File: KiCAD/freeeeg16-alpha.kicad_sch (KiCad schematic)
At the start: 27 parts, among them J1 Conn_02x03_Odd_Even, J2 Conn_01x03, J28 Conn_02x03_Odd_Even, J29 Conn_02x03_Odd_Even, J3 Conn_01x03, J30 Conn_02x03_Odd_Even, J31 Conn_02x03_Odd_Even, J32 Conn_02x03_Odd_Even, J33 Conn_02x03_Odd_Even, J5 Conn_01x08, J6 Conn_01x06, SW1 SW_Push, SW2 SW_Push, SW3 SW_Push, SW4 SW_Push

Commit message: Add files via upload
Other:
- moved on the sheet: C20, C39, C41, J1, J2, J3, J5, J6, R1, R10, R2, R4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

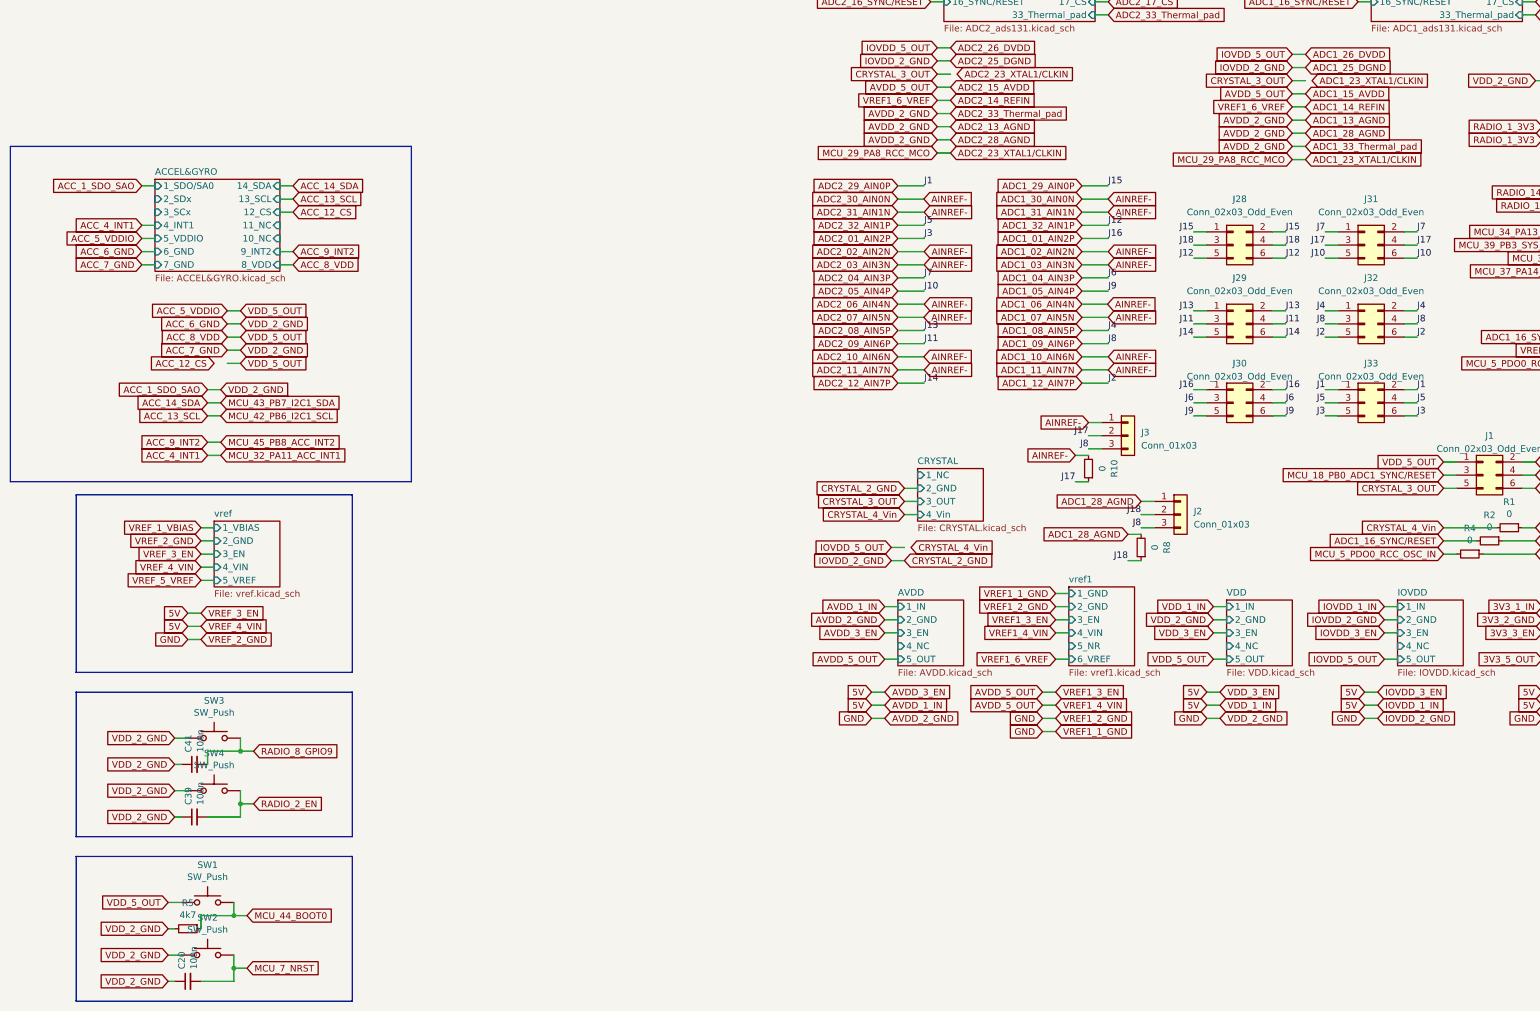
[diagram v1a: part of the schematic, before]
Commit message: Add files via upload
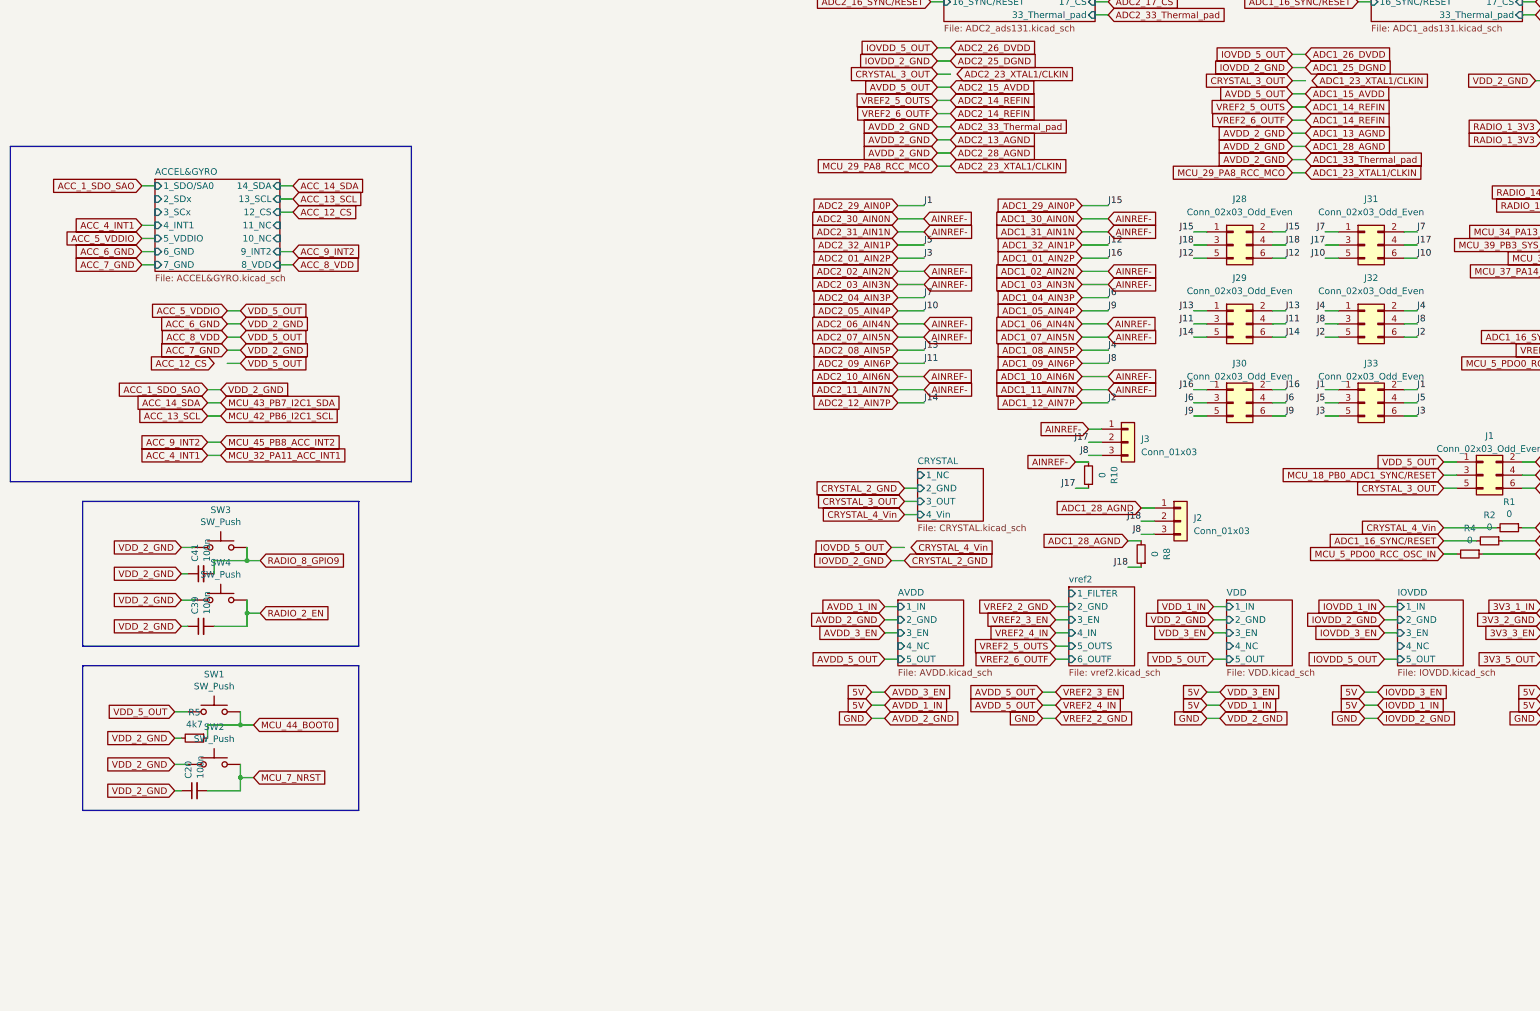
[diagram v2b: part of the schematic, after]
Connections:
- net ADC1_14_REFIN: no longer J6.4 (Pin_4)
- new net VREF1_6_VREF: J6.4 (Pin_4)
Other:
- removed sheet vref
- removed sheet vref1
- added sheet vref2 (vref2.kicad_sch)
- moved on the sheet: C20, C39, C41, J2, J3, R10, R5, R8, SW1, SW2, SW3, SW4

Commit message: Add files via upload
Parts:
- added R13: 10k, Resistor_SMD:R_0402_1005Metric, symbol FreeEEG32-ads131-rescue:R_Small-Device
- C39: value 100n -> 1u; MNP CL05B104KO5NNNC -> CL05A105KO5NNNC
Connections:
- net VREF1_6_VREF is gone; now on net ADC1_14_REFIN: J6.4 (Pin_4)
- net 3V3_5_OUT: now also R13.2
- net RADIO_2_EN: now also R13.1
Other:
- moved on the sheet: C20, C39, C41, R5, SW1, SW2, SW3, SW4
